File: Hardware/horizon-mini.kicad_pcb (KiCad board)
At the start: 2 copper layers, 34 x 41.8 mm, 89 parts, among them J1 Screw_Terminal_01x02, J16 arming terminal, J2 Screw_Terminal_01x02, J3 Micro_SD_Card_Det1, J7 USB_C_Receptacle_USB2.0_16P, J8 Conn_02x03_Counter_Clockwise, Q1 BSS138, Q10 DMG2301L, Q2 IRLML6402, U1 TPS82130, U16 AP2112K-3.3, U2 TPS61092, U3 LTC4412xS6, U5 ATSAMD21G18A-A, U6 NAND, U7 LPS22HB, U9 LSM6DS3

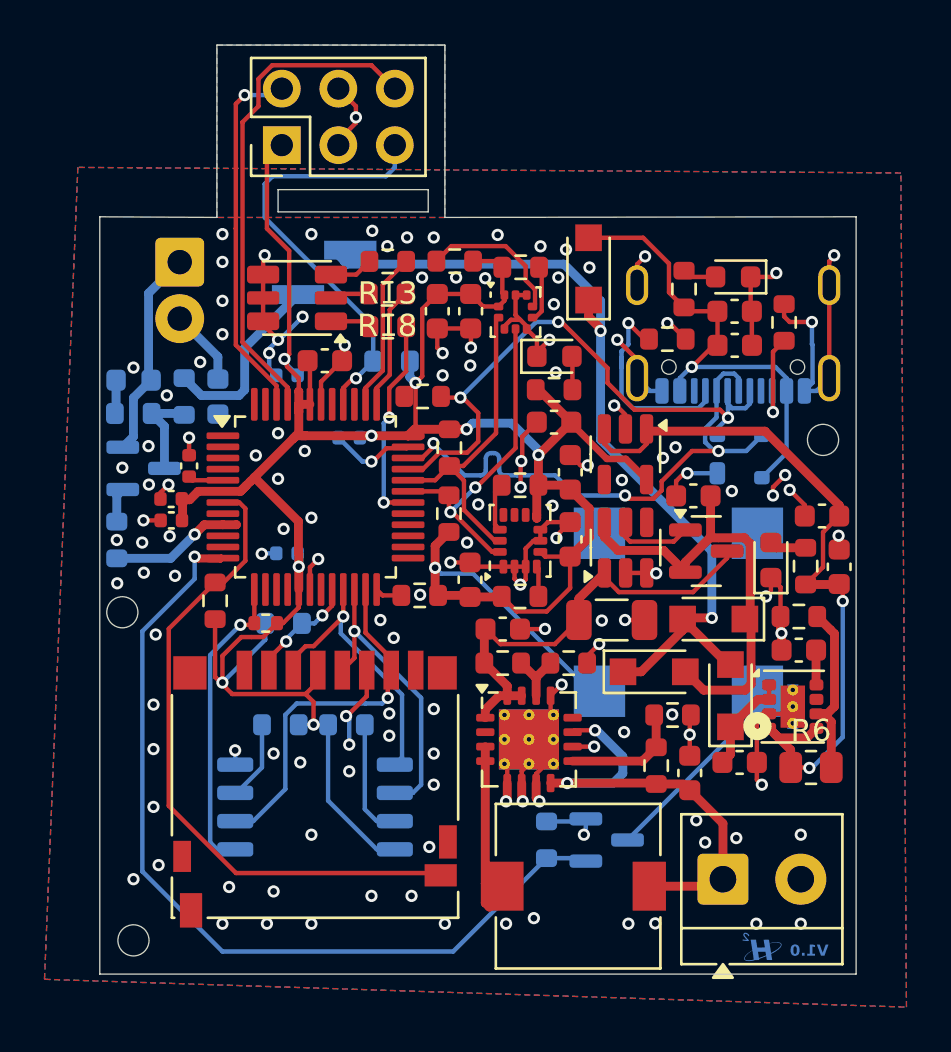
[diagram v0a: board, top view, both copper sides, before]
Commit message: forgot to push from last night. Very small silscreen changes and stuff
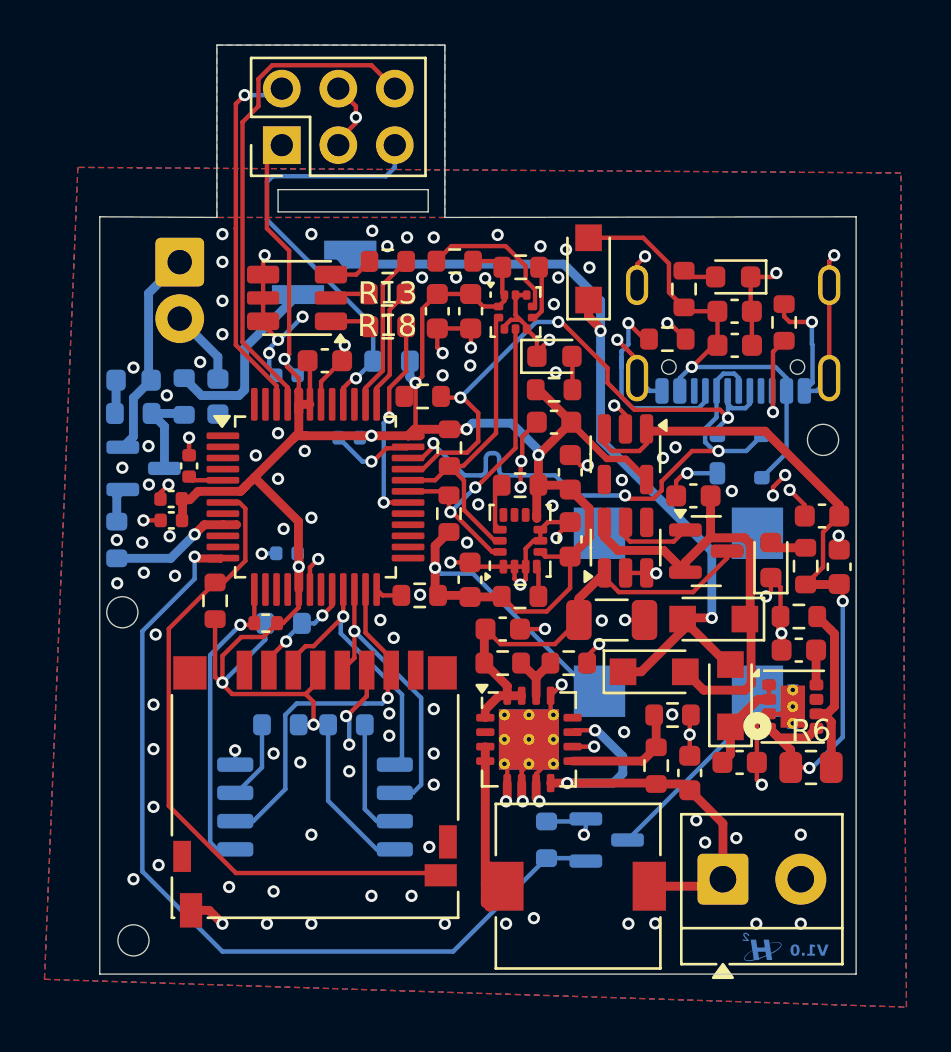
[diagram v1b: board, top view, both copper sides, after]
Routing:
- net GND: track 106.1 -> 107.8 mm
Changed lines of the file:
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@@
 	)
 	(segment
+		(start 140.0875 133.65)
+		(end 140.9 133.65)
+		(width 0.4)
+		(layer "F.Cu")
+		(net 2)
+	)
+	(segment
 		(start 157.922345 113.64601)
 		(end 157.600931 113.64601)
@@
 	)
 	(segment
+		(start 140.9 133.65)
+		(end 141.5 134.25)
+		(width 0.4)
+		(layer "F.Cu")
+		(net 2)
+	)
+	(segment
 		(start 156.253661 124.740007)
 		(end 156.378661 124.865007)
@@
 	)
 	(segment
-		(start 148.851 100.649)
-		(end 149.25 100.25)
+		(start 143.501292 100.898766)
+		(end 143.751058 100.649)
 		(width 0.2)
 		(layer "B.Cu")
@@
 	)
 	(segment
-		(start 148.275746 107.375688)
-		(end 143.399 102.498942)
+		(start 149.25 100.25)
+		(end 149.25 99.25)
 		(width 0.2)
 		(layer "B.Cu")
@@
 	)
 	(segment
-		(start 149.25 100.25)
-		(end 149.25 99.25)
+		(start 148.851 100.649)
+		(end 149.25 100.25)
 		(width 0.2)
 		(layer "B.Cu")
@@
 	)
 	(segment
-		(start 143.399 102.498942)
-		(end 143.399 101.001058)
+		(start 148.275746 107.375688)
+		(end 143.501292 102.601234)
 		(width 0.2)
 		(layer "B.Cu")
@@
 	)
 	(segment
-		(start 147.504561 109.732048)
-		(end 148.275746 108.960863)
+		(start 148.275746 108.960863)
+		(end 148.275746 107.375688)
 		(width 0.2)
 		(layer "B.Cu")
@@
 	)
 	(segment
-		(start 143.399 101.001058)
-		(end 143.751058 100.649)
+		(start 143.751058 100.649)
+		(end 148.851 100.649)
 		(width 0.2)
 		(layer "B.Cu")
@@
 	)
 	(segment
-		(start 148.275746 108.960863)
-		(end 148.275746 107.375688)
+		(start 147.504561 109.732048)
+		(end 148.275746 108.960863)
 		(width 0.2)
 		(layer "B.Cu")
@@
 	)
 	(segment
-		(start 143.751058 100.649)
-		(end 148.851 100.649)
+		(start 143.501292 102.601234)
+		(end 143.501292 100.898766)
 		(width 0.2)
 		(layer "B.Cu")
@@
 	)
 	(segment
-		(start 137.899 131.899)
-		(end 137.899 121.101)
+		(start 140.25 118.75)
+		(end 140.25 117.75)
 		(width 0.2)
 		(layer "B.Cu")
@@
 	)
 	(segment
-		(start 140.25 118.75)
-		(end 140.25 117.75)
+		(start 156.070027 131.303671)
+		(end 151.873698 135.5)
 		(width 0.2)
 		(layer "B.Cu")
@@
 	)
 	(segment
-		(start 137.899 121.101)
-		(end 140.25 118.75)
+		(start 137.899 131.899)
+		(end 137.899 121.101)
 		(width 0.2)
 		(layer "B.Cu")
@@
 	)
 	(segment
-		(start 151.873698 135.5)
-		(end 141.5 135.5)
+		(start 137.899 121.101)
+		(end 140.25 118.75)
 		(width 0.2)
 		(layer "B.Cu")
@@
 	)
 	(segment
-		(start 156.070027 131.303671)
-		(end 151.873698 135.5)
+		(start 151.873698 135.5)
+		(end 141.5 135.5)
 		(width 0.2)
 		(layer "B.Cu")
@@
 		(polygon
 			(pts
-				(xy 164.98089 134.149071) (xy 169.180475 134.149071) (xy 169.221953 136.010369) (xy 164.322437 136.020738)
-				(xy 164.363914 134.154256) (xy 164.99126 134.154256)
+				(xy 164.98089 134.149071) (xy 169.25 134.149071) (xy 169.25 136.25) (xy 164.322437 136.25) (xy 164.363914 134.154256)
+				(xy 164.99126 134.154256)
 			)
 		)
